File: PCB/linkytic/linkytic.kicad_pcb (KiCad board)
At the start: 2 copper layers, 29.5 x 57 mm, 14 parts, among them J1 L2, J2 L1, J3 A, SW1 benoit, U1 M5333B, U2 E18-MS1-PCB, U3 CC_debugger

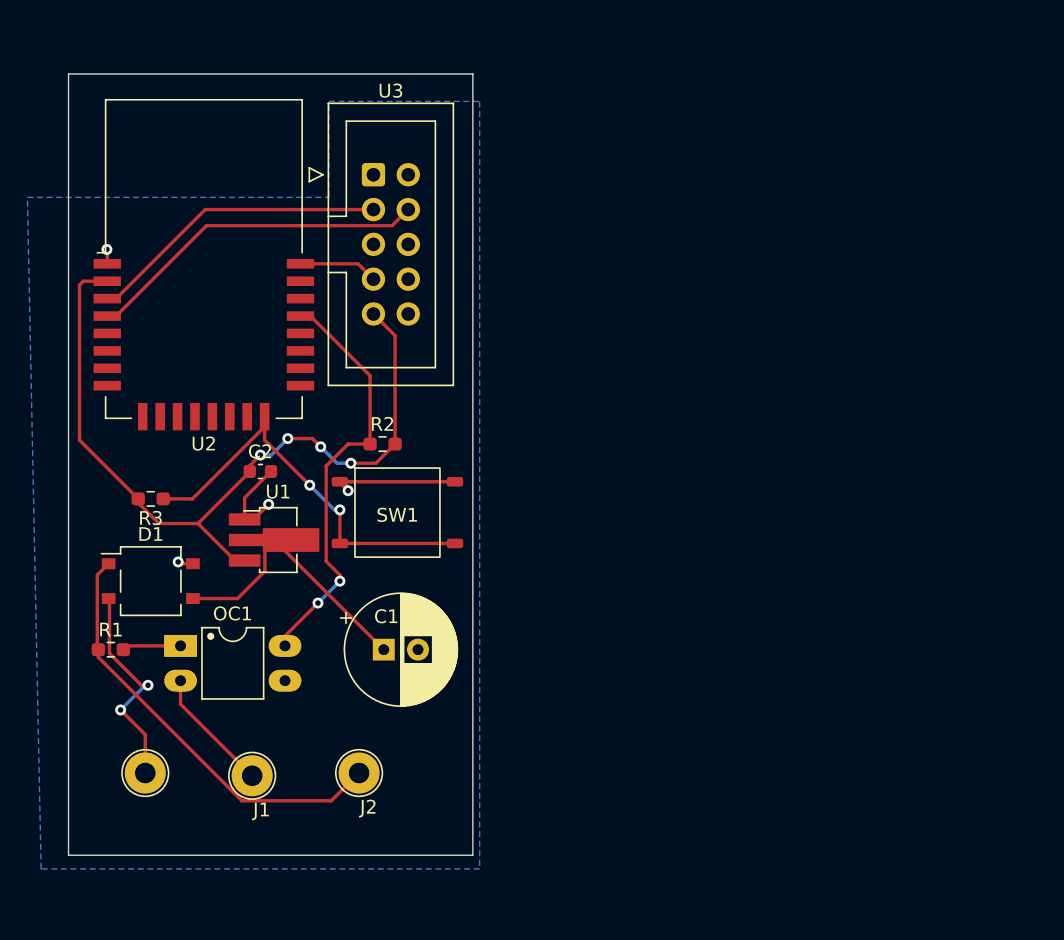
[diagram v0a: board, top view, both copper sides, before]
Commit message: Update final version V0
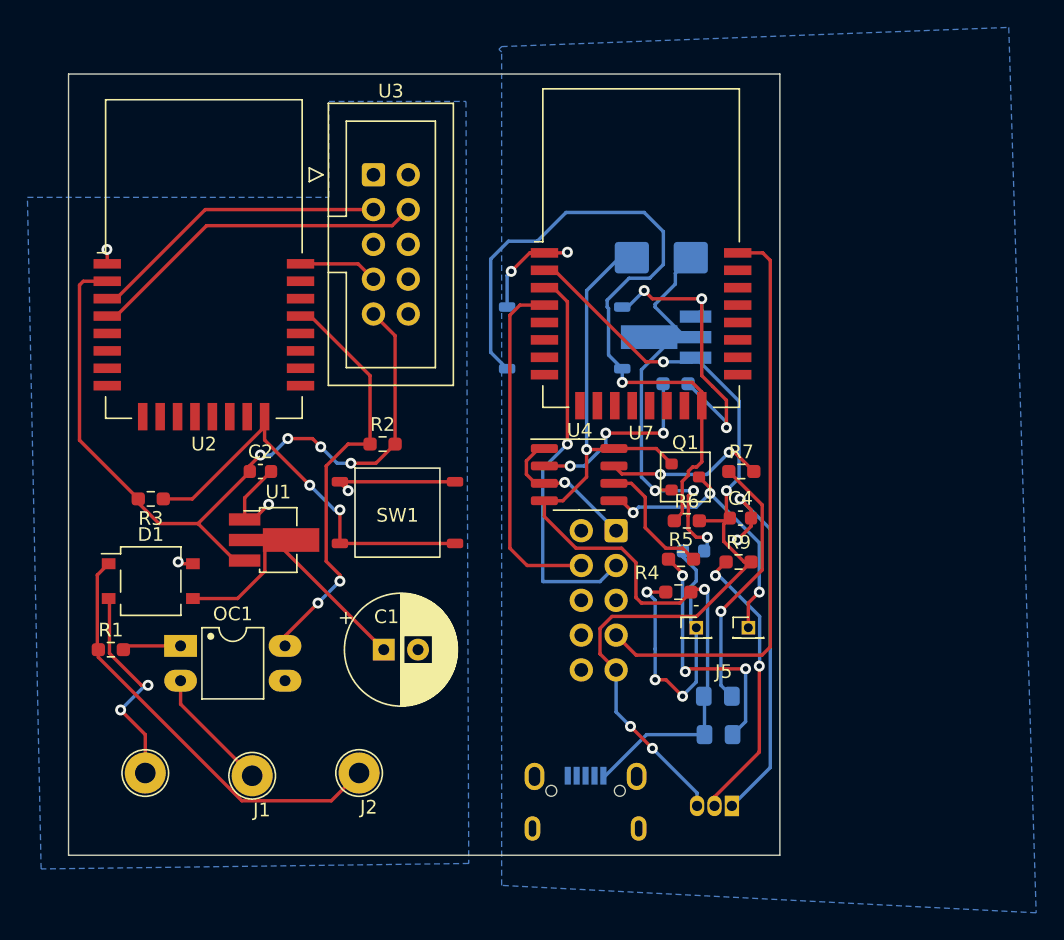
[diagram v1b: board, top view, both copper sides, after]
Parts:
- added -: BAT-, Connector_PinHeader_1.27mm:PinHeader_1x01_P1.27mm_Vertical, F.Cu at (88.8, 78.4)
- added C3: 1u, Capacitor_SMD:C_0603_1608Metric, B.Cu at (88.6, 72.8)
- added C4: 10uF, Capacitor_SMD:C_0603_1608Metric, F.Cu at (92.0, 70.4)
- added D2: GREENLED, LED_SMD:LED_0805_2012Metric_Pad1.15x1.40mm_HandSolder, B.Cu at (90.4, 86.2)
- added D3: REDLED, LED_SMD:LED_0805_2012Metric_Pad1.15x1.40mm_HandSolder, B.Cu at (90.4, 83.4)
- added D4: SS24, Diode_SMD_AKL:D_SMB, B.Cu at (86.2, 51.4)
- added J5: BAT+, Connector_PinHeader_1.27mm:PinHeader_1x01_P1.27mm_Vertical, F.Cu at (92.6, 78.4)
- added J6: USB_B_Micro, usb:USB_aliexpress, B.Cu at (79.4, 87.2)
- added Q1: AO3407A, Package_TO_SOT_SMD_AKL:SOT-23, F.Cu at (88.0, 67.4)
- added R4: 100k, Resistor_SMD:R_0603_1608Metric_Pad0.98x0.95mm_HandSolder, F.Cu at (87.5, 75.8)
- added R5: 1k, Resistor_SMD:R_0603_1608Metric_Pad0.98x0.95mm_HandSolder, F.Cu at (87.7, 73.4)
- added R6: 10k, Resistor_SMD:R_0603_1608Metric_Pad0.98x0.95mm_HandSolder, F.Cu at (88.1, 70.6)
- added R7: 1k, Resistor_SMD:R_0603_1608Metric_Pad0.98x0.95mm_HandSolder, F.Cu at (92.1, 67.0)
- added R8: 1.2k, Resistor_SMD:R_0603_1608Metric_Pad0.98x0.95mm_HandSolder, B.Cu at (87.3, 60.6)
- added R9: 10k, Resistor_SMD:R_0603_1608Metric_Pad0.98x0.95mm_HandSolder, F.Cu at (91.9, 73.6)
- added SW2: benoit2, Library:interrupteur, B.Cu at (83.4, 55.0)
- added U4: TP4056, Package_SO:SOP-8_3.76x4.96mm_P1.27mm, F.Cu at (80.3, 67.2)
- added U5: M5333B, Package_TO_SOT_SMD:SOT-89-3_Handsoldering, B.Cu at (86.6, 57.2)
- added U6: CC_debugger, Connector_IDC:IDC-Header_2x05_P2.54mm_Vertical, B.Cu at (83.0, 71.3)
- added U7: E18-MS1-PCB, RF_Module:E18-MS1-PCB, F.Cu at (84.8, 50.7)
- added U8: DS18B20, Package_TO_SOT_THT:TO-92_Inline, B.Cu at (91.4, 91.4)
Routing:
- net GND_2: track 0.00 -> 91.3 mm, vias 0 -> 11
- net USB_IN: track 0.00 -> 65.3 mm, vias 0 -> 2
- net VDD2: track 0.00 -> 63.1 mm, vias 0 -> 4
- net Net-(R6-Pad1): track 0.00 -> 53.6 mm, vias 0 -> 1
- net Net-(U6-Pad7): track 0.00 -> 42.9 mm
- net Net-(D4-Pad1): track 0.00 -> 32.3 mm, vias 0 -> 3
- net Net-(U6-Pad3): track 0.00 -> 29.1 mm, vias 0 -> 1
- net Net-(U6-Pad4): track 0.00 -> 25.6 mm
- net Net-(J5-Pad1): track 0.00 -> 21.1 mm, vias 0 -> 3
- net Net-(R9-Pad1): track 0.00 -> 21.0 mm, vias 0 -> 2
- net Net-(D3-Pad1): track 0.00 -> 19.0 mm, vias 0 -> 1
- net Net-(D2-Pad1): track 0.00 -> 18.4 mm, vias 0 -> 3
- net Net-(R8-Pad2): track 0.00 -> 13.8 mm, vias 0 -> 3
- net Net-(R7-Pad2): track 0.00 -> 11.7 mm, vias 0 -> 2
- net Net-(R5-Pad2): track 0.00 -> 9.40 mm
- added copper zone on B.Cu, net GND_2
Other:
- board size 29.5 x 57 mm -> 51.9 x 57 mm
- board text added: "LINKYTIC MBE V0"
- board text added: "Zigbee Thermometer V0 MBE"
